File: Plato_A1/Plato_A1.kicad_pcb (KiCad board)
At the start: 2 copper layers, 31 x 35.6 mm, 23 parts, among them J1 Conn_01x03_Socket, J2 Conn_01x03_Pin

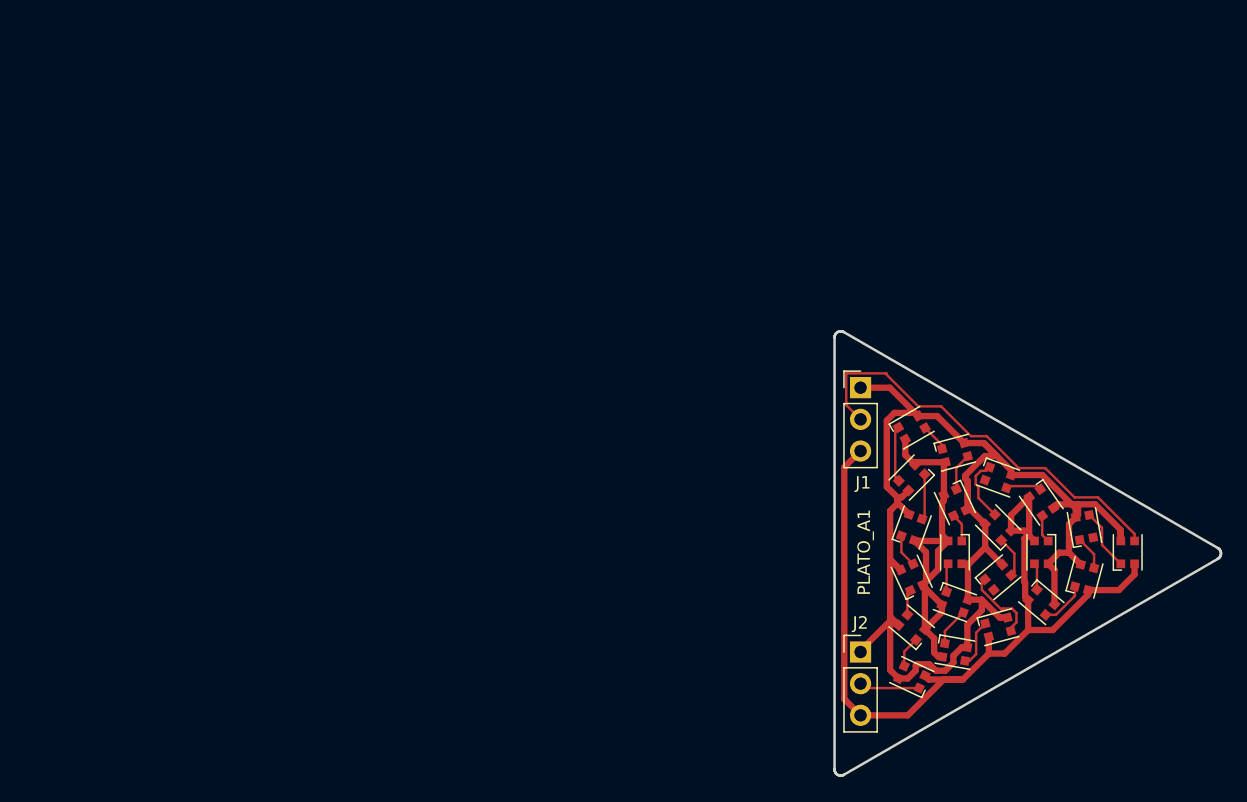
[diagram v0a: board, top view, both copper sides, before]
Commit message: Abortative redesign
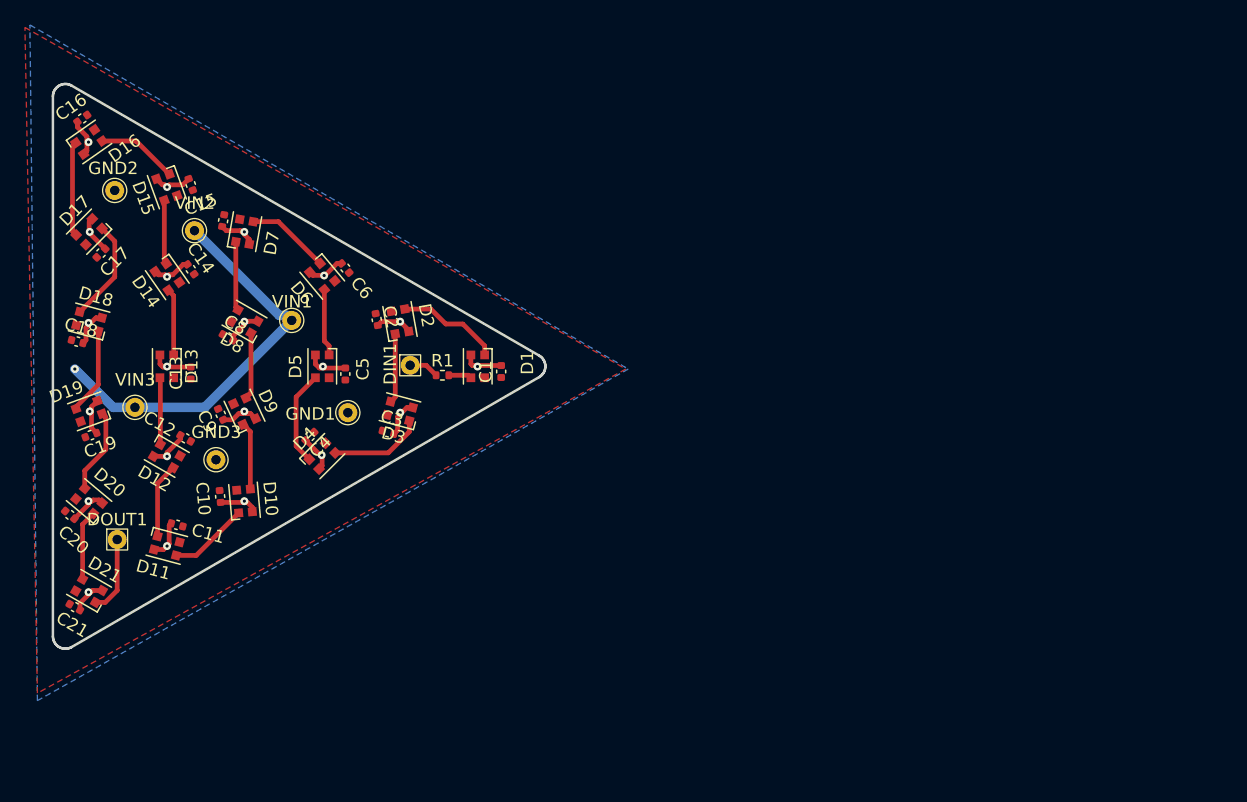
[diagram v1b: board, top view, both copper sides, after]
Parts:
- removed J1: Conn_01x03_Socket, Connector_PinHeader_2.54mm:PinHeader_1x03_P2.54mm_Vertical
- removed J2: Conn_01x03_Pin, Connector_PinHeader_2.54mm:PinHeader_1x03_P2.54mm_Vertical
- added C1: 100nF, Capacitor_SMD:C_0402_1005Metric, F.Cu at (70.8, 58.0)
- added C10: 100nF, Capacitor_SMD:C_0402_1005Metric, F.Cu at (48.3, 68.0)
- added C11: 100nF, Capacitor_SMD:C_0402_1005Metric, F.Cu at (44.8, 70.3)
- added C12: 100nF, Capacitor_SMD:C_0402_1005Metric, F.Cu at (45.5, 63.4)
- added C13: 100nF, Capacitor_SMD:C_0402_1005Metric, F.Cu at (45.9, 58.1)
- added C14: 100nF, Capacitor_SMD:C_0402_1005Metric, F.Cu at (45.9, 49.8)
- added C15: 100nF, Capacitor_SMD:C_0402_1005Metric, F.Cu at (45.9, 43.0)
- added C16: 100nF, Capacitor_SMD:C_0402_1005Metric, F.Cu at (37.2, 37.7)
- added C17: 100nF, Capacitor_SMD:C_0402_1005Metric, F.Cu at (38.7, 48.5)
- added C18: 100nF, Capacitor_SMD:C_0402_1005Metric, F.Cu at (36.8, 55.6)
- added C19: 100nF, Capacitor_SMD:C_0402_1005Metric, F.Cu at (37.9, 63.1)
- added C2: 100nF, Capacitor_SMD:C_0402_1005Metric, F.Cu at (60.8, 53.8)
- added C20: 100nF, Capacitor_SMD:C_0402_1005Metric, F.Cu at (36.2, 69.5)
- added C21: 100nF, Capacitor_SMD:C_0402_1005Metric, F.Cu at (36.6, 76.9)
- added C3: 100nF, Capacitor_SMD:C_0402_1005Metric, F.Cu at (61.7, 62.9)
- added C4: 100nF, Capacitor_SMD:C_0402_1005Metric, F.Cu at (55.5, 63.2)
- added C5: 100nF, Capacitor_SMD:C_0402_1005Metric, F.Cu at (58.3, 58.2)
- added C6: 100nF, Capacitor_SMD:C_0402_1005Metric, F.Cu at (58.3, 49.7)
- added C7: 100nF, Capacitor_SMD:C_0402_1005Metric, F.Cu at (48.5, 45.9)
- added C8: 100nF, Capacitor_SMD:C_0402_1005Metric, F.Cu at (48.9, 55.3)
- added C9: 100nF, Capacitor_SMD:C_0402_1005Metric, F.Cu at (48.3, 61.4)
- added DIN1: Conn_01x01, Library:DataHole, F.Cu at (63.5, 57.5)
- added DOUT1: Conn_01x01, Library:DataHole, F.Cu at (40.0, 71.5)
- added GND1: Conn_01x01, Library:PowerHole, F.Cu at (58.5, 61.3)
- added GND2: Conn_01x01, Library:PowerHole, F.Cu at (39.8, 43.5)
- added GND3: Conn_01x01, Library:PowerHole, F.Cu at (47.9, 65.1)
- added R1: 330ohm, Resistor_SMD:R_0402_1005Metric, F.Cu at (66.1, 58.3)
- added VIN1: Conn_01x01, Library:PowerHole, F.Cu at (54.0, 53.9)
- added VIN2: Conn_01x01, Library:PowerHole, F.Cu at (46.2, 46.7)
- added VIN3: Conn_01x01, Library:PowerHole, F.Cu at (41.4, 60.9)
- moved D16 69.9 mm to (37.7, 39.6), turned to 35 degrees
- moved D17 68.9 mm to (37.7, 46.8)
- moved D18 68.0 mm to (37.7, 54.0), turned to 165 degrees
- moved D19 67.3 mm to (37.7, 61.2), turned to -160 degrees
- moved D20 66.8 mm to (37.7, 68.4)
- moved D15 66.7 mm to (44.0, 43.2), turned to -70 degrees
- moved D21 66.4 mm to (37.7, 75.6), turned to 150 degrees
- moved D14 65.7 mm to (44.0, 50.4), turned to -55 degrees
- moved D13 65.0 mm to (44.0, 57.6)
- moved D12 64.3 mm to (44.0, 64.8), turned to -30 degrees
- moved D11 63.8 mm to (44.0, 72.0), turned to -15 degrees
- moved D7 63.6 mm to (50.2, 46.8), turned to 80 degrees
- moved D8 62.7 mm to (50.2, 54.0), turned to 150 degrees
- moved D9 61.9 mm to (50.2, 61.2), turned to 115 degrees
- moved D10 61.3 mm to (50.2, 68.4), turned to 95 degrees
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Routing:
- net +5V: track 111.1 -> 32.3 mm, vias 0 -> 1
- net GND: track 105.2 -> 65.4 mm, vias 0 -> 21
- net DATA_IN: track 33.3 -> 1.85 mm
- net Net-(D4-DOUT): track 2.16 -> 7.62 mm
- net Net-(D19-DOUT): track 2.03 -> 6.81 mm
- net Net-(D17-DOUT): track 3.67 -> 8.28 mm
- net Net-(D18-DOUT): track 2.66 -> 6.97 mm
- net Net-(D15-DOUT): track 2.25 -> 6.48 mm
- net Net-(D6-DOUT): track 2.88 -> 6.76 mm
- net Net-(D3-DOUT): track 3.72 -> 7.53 mm
- net Net-(D1-DOUT): track 4.96 -> 8.36 mm
- net Net-(D5-DOUT): track 2.22 -> 5.39 mm
- net Net-(D20-DOUT): track 2.50 -> 5.61 mm
- net Net-(D16-DOUT): track 4.50 -> 7.61 mm
- net Net-(D13-DOUT): track 2.30 -> 5.37 mm
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- added copper zone on F.Cu, net +5V
- added copper zone on B.Cu, net GND
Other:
- board size 31 x 35.6 mm -> 39.5 x 45.3 mm
- board text removed: "5V"
- board text removed: "DIN"
- board text removed: "DOUT"
- board text removed: "GND"
- board text removed: "PLATO_A1"
- board text removed: "PLATO_A1 APRIL 12024 SZC SUPERLUMINOUS https://github.com/koopero/Plato JLCJLCJLCJLC"

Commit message: Restore final product
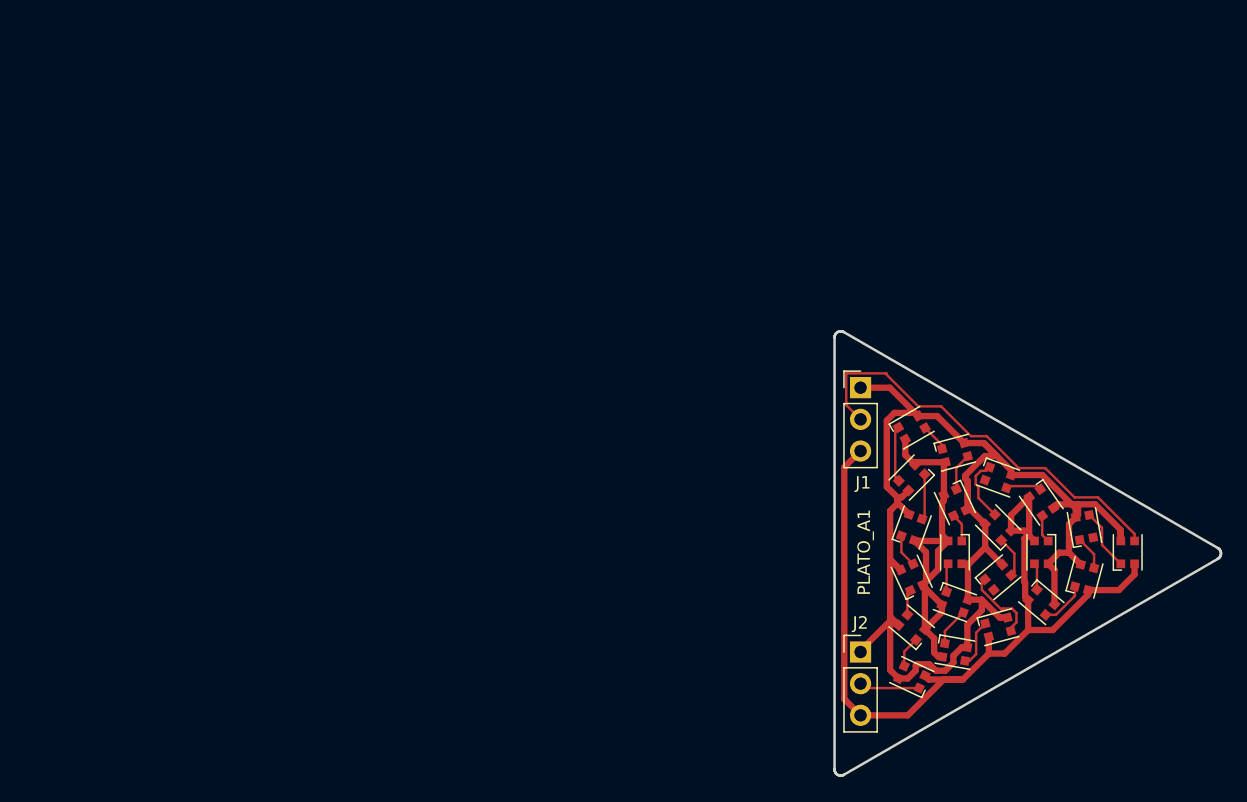
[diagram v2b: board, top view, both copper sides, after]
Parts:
- removed C1, C10, C11, C12, C13, C14, C15, C16, C17, C18, C19, C2, C20, C21, C3, C4, C5, C6, C7, C8, C9: 100nF, Capacitor_SMD:C_0402_1005Metric
- removed DIN1, DOUT1: Conn_01x01, Library:DataHole
- removed GND1, GND2, GND3, VIN1, VIN2, VIN3: Conn_01x01, Library:PowerHole
- removed R1: 330ohm, Resistor_SMD:R_0402_1005Metric
- added J1: Conn_01x03_Socket, Connector_PinHeader_2.54mm:PinHeader_1x03_P2.54mm_Vertical, F.Cu at (99.6, 59.3)
- added J2: Conn_01x03_Pin, Connector_PinHeader_2.54mm:PinHeader_1x03_P2.54mm_Vertical, F.Cu at (99.6, 80.5)
- moved D16 69.9 mm to (103.7, 62.5), turned to 30 degrees
- moved D17 68.9 mm to (103.7, 66.5)
- moved D18 68.0 mm to (103.7, 70.5), turned to 70 degrees
- moved D19 67.3 mm to (103.7, 74.5), turned to 115 degrees
- moved D20 66.8 mm to (103.7, 78.5)
- moved D15 66.7 mm to (107.2, 64.5), turned to 15 degrees
- moved D21 66.4 mm to (103.7, 82.5), turned to 155 degrees
- moved D14 65.7 mm to (107.2, 68.5), turned to -65 degrees
- moved D13 65.0 mm to (107.2, 72.5)
- moved D12 64.3 mm to (107.2, 76.5), turned to -20 degrees
- moved D11 63.8 mm to (107.2, 80.5), turned to -10 degrees
- moved D7 63.6 mm to (110.7, 66.5), turned to -20 degrees
- moved D8 62.7 mm to (110.7, 70.5), turned to 135 degrees
- moved D9 61.9 mm to (110.7, 74.5), turned to 40 degrees
- moved D10 61.3 mm to (110.7, 78.5), turned to 15 degrees
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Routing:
- net +5V: track 32.3 -> 111.1 mm, vias 1 -> 0
- net GND: track 65.4 -> 105.2 mm, vias 21 -> 0
- net DATA_IN: track 1.85 -> 33.3 mm
- net Net-(D4-DOUT): track 7.62 -> 2.16 mm
- net Net-(D19-DOUT): track 6.81 -> 2.03 mm
- net Net-(D17-DOUT): track 8.28 -> 3.67 mm
- net Net-(D18-DOUT): track 6.97 -> 2.66 mm
- net Net-(D15-DOUT): track 6.48 -> 2.25 mm
- net Net-(D6-DOUT): track 6.76 -> 2.88 mm
- net Net-(D3-DOUT): track 7.53 -> 3.72 mm
- net Net-(D1-DOUT): track 8.36 -> 4.96 mm
- net Net-(D5-DOUT): track 5.39 -> 2.22 mm
- net Net-(D20-DOUT): track 5.61 -> 2.50 mm
- net Net-(D16-DOUT): track 7.61 -> 4.50 mm
- net Net-(D13-DOUT): track 5.37 -> 2.30 mm
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- removed copper zone on F.Cu, net +5V
- removed copper zone on B.Cu, net GND
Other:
- board size 39.5 x 45.3 mm -> 31 x 35.6 mm
- board text added: "5V"
- board text added: "DIN"
- board text added: "DOUT"
- board text added: "GND"
- board text added: "PLATO_A1"
- board text added: "PLATO_A1 APRIL 12024 SZC SUPERLUMINOUS https://github.com/koopero/Plato JLCJLCJLCJLC"
